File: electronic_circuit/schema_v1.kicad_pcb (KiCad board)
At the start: 2 copper layers, 74.2 x 51.8 mm, 34 parts, among them J1 Screw_Terminal_1x02, Q1 BC547, Q2 BC547, Q3 BC547, Q4 BC547, U1 MosfetIRF, U2 MosfetIRF, U3 STM32-Nucleo_Pinout, U4 MosfetIRF, U5 MosfetIRF, U6 mrf24j40ma, U7 DS-001

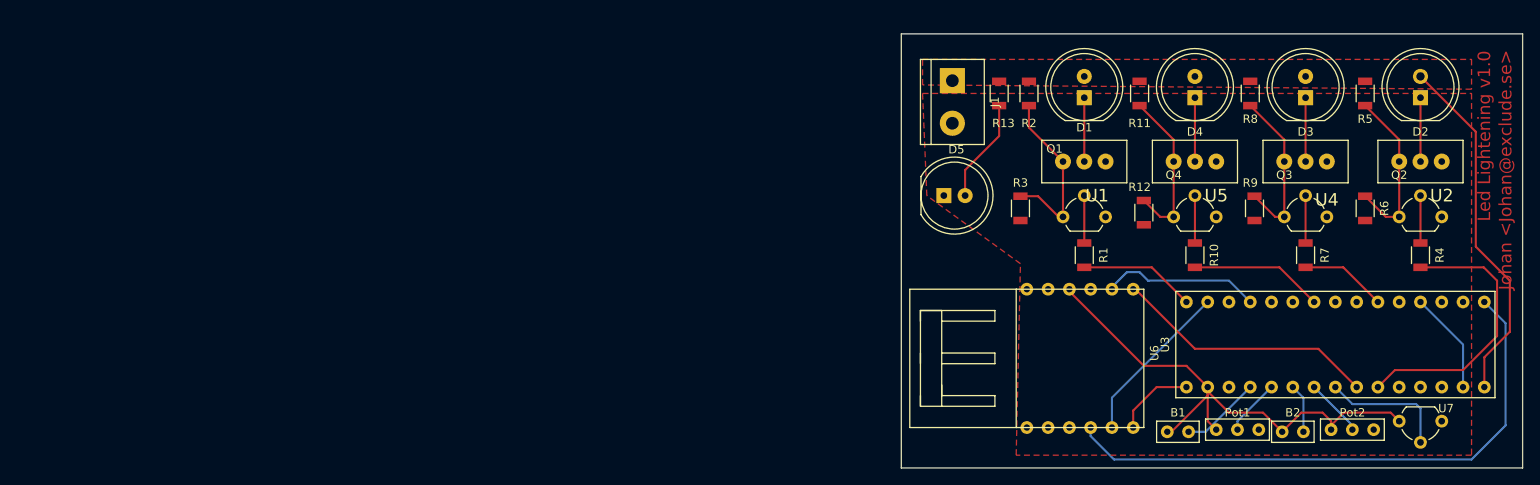
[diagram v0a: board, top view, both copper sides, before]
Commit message: New electronic schema
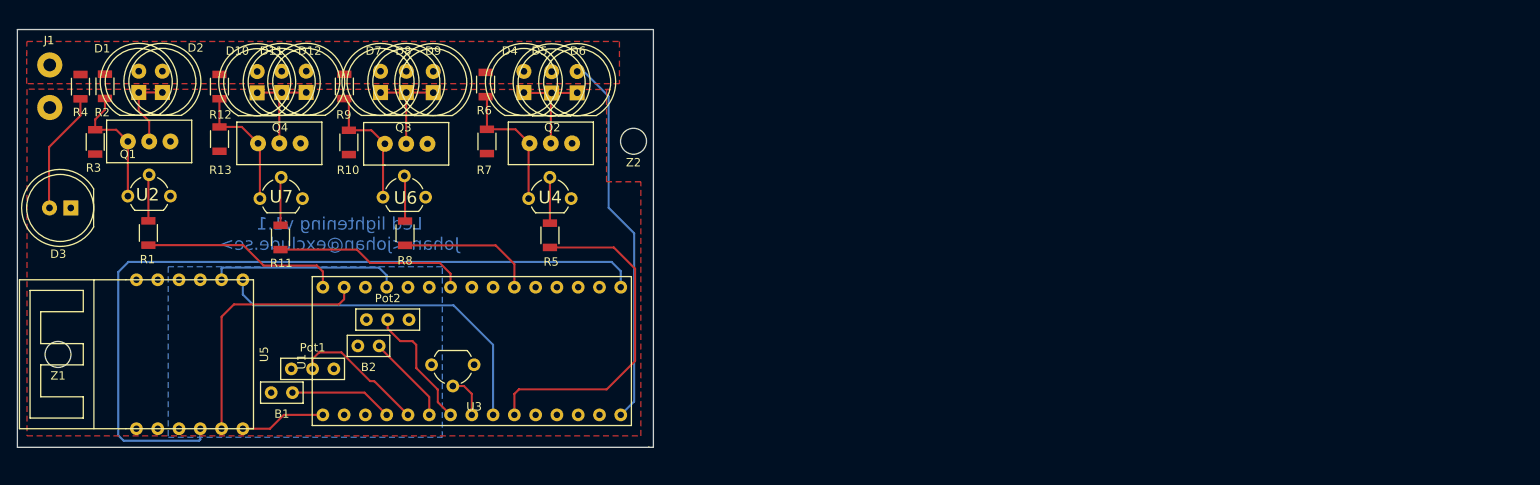
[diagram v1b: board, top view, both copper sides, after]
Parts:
- added D10: LED, LEDs:LED-8MM, F.Cu at (63.3, 30.4)
- added D11: LED, LEDs:LED-8MM, F.Cu at (69.2, 30.4)
- added D12: LED, LEDs:LED-8MM, F.Cu at (66.2, 30.4)
- added D6: LED, LEDs:LED-8MM, F.Cu at (101.5, 30.4)
- added D7: LED, LEDs:LED-8MM, F.Cu at (78.0, 30.4)
- added D8: LED, LEDs:LED-8MM, F.Cu at (81.1, 30.4)
- added D9: LED, LEDs:LED-8MM, F.Cu at (84.3, 30.4)
- added Z1: Drill_Hole, DrillHole:Drill_Hole, F.Cu at (39.5, 59.1)
- added Z2: Drill_Hole, DrillHole:Drill_Hole, F.Cu at (108.2, 33.6)
- J1: footprint Connectors:bornier2 -> potHoles:P_Led_Holes
- R10, R7: value 1k -> 39k
- R11, R5, R8: value 12k -> 1k
- R12, R6, R9: value 39k -> 12k
- R13: value 12k -> 39k
- R4: value 1k -> 12k
- U1: value MosfetIRF -> STM32-Nucleo_Pinout; footprint library:IRF3205 -> stm32nucleo:STM32-Nucleo_Pinout
- U3: value STM32-Nucleo_Pinout -> DS-001; footprint stm32nucleo:STM32-Nucleo_Pinout -> TO_SOT_Packages_THT:TO-92_Molded_Wide
- U5: value MosfetIRF -> mrf24j40ma; footprint library:IRF3205 -> mrf24j40ma:mrf24j40ma
- U6: value mrf24j40ma -> MosfetIRF; footprint mrf24j40ma:mrf24j40ma -> library:IRF3205
- U7: value DS-001 -> MosfetIRF; footprint TO_SOT_Packages_THT:TO-92_Molded_Wide -> library:IRF3205
- moved R4 161.2 mm to (42.2, 29.7)
- moved U2 151.8 mm to (47.9, 36.2)
- moved D2 150.2 mm to (52.0, 30.4)
- moved D3 148.0 mm to (41.1, 44.1), turned to 180 degrees
- moved U7 145.1 mm to (63.4, 36.4), turned to 0 degrees
- moved U5 139.7 mm to (34.9, 61.6), turned to 90 degrees
- moved U3 123.2 mm to (89.2, 62.9), turned to 180 degrees
- moved Pot2 115.4 mm to (78.9, 60.0), turned to 180 degrees
- moved D1 112.9 mm to (49.2, 30.4)
- moved R1 111.8 mm to (50.3, 47.1)
- moved Q1 111.7 mm to (47.9, 42.7)
- moved R12 111.4 mm to (58.8, 29.7)
- moved B2 110.8 mm to (76.6, 59.3)
- moved R3 110.7 mm to (44.0, 36.3)
- moved Pot1 110.4 mm to (69.9, 65.9), turned to 180 degrees
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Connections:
- D2 pad 1: Net-(D2-Pad1) -> Net-(D1-Pad1)
- D3 pad 1: Net-(D3-Pad1) -> GNDREF
- D3 pad 2: 12V -> Net-(D3-Pad2)
- D5 pad 1: GNDREF -> Net-(D4-Pad1)
- D5 pad 2: Net-(D5-Pad2) -> 12V
- R10 pad 1: Net-(Q4-Pad2) -> Net-(Q3-Pad1)
- R10 pad 2: RGB_B -> GNDREF
- R11 pad 1: 12V -> Net-(Q4-Pad2)
- R11 pad 2: Net-(Q4-Pad1) -> RGB_B
- R12 pad 1: Net-(Q4-Pad1) -> 12V
- R12 pad 2: GNDREF -> Net-(Q4-Pad1)
- R13 pad 1: 12V -> Net-(Q4-Pad1)
- R13 pad 2: Net-(D5-Pad2) -> GNDREF
- R4 pad 1: Net-(Q2-Pad2) -> 12V
- R4 pad 2: RGB_R -> Net-(D3-Pad2)
- R5 pad 1: 12V -> Net-(Q2-Pad2)
- R5 pad 2: Net-(Q2-Pad1) -> RGB_R
- R6 pad 1: Net-(Q2-Pad1) -> 12V
- R6 pad 2: GNDREF -> Net-(Q2-Pad1)
- R7 pad 1: Net-(Q3-Pad2) -> Net-(Q2-Pad1)
- R7 pad 2: RGB_G -> GNDREF
- R8 pad 1: 12V -> Net-(Q3-Pad2)
- R8 pad 2: Net-(Q3-Pad1) -> RGB_G
- R9 pad 1: Net-(Q3-Pad1) -> 12V
- R9 pad 2: GNDREF -> Net-(Q3-Pad1)
- U1 pad 1: Net-(Q1-Pad1) -> SPI_INT
- U1 pad 2: Net-(D1-Pad1) -> Net-(U1-Pad2)
- U1 pad 3: GNDREF -> Net-(U1-Pad3)
- U2 pad 1: Net-(Q2-Pad1) -> Net-(Q1-Pad1)
- U2 pad 2: Net-(D2-Pad1) -> Net-(D1-Pad1)
- U3 pad 1: SPI_INT -> GNDREF
- U3 pad 2: Net-(U3-Pad2) -> TEMP_SENSOR
- U3 pad 3: Net-(U3-Pad3) -> 3.3V
- U4 pad 1: Net-(Q3-Pad1) -> Net-(Q2-Pad1)
- U4 pad 2: Net-(D3-Pad1) -> Net-(D4-Pad1)
- U5 pad 1: Net-(Q4-Pad1) -> GNDREF
- U5 pad 2: Net-(D4-Pad1) -> MRF_RESET
- U5 pad 3: GNDREF -> Net-(U5-Pad3)
- U6 pad 1: GNDREF -> Net-(Q3-Pad1)
- U6 pad 3: MRF_RESET -> GNDREF
- U7 pad 1: GNDREF -> Net-(Q4-Pad1)
- U7 pad 2: TEMP_SENSOR -> Net-(D10-Pad1)
- U7 pad 3: 3.3V -> GNDREF
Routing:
- net 3.3V: track 63.9 -> 0.00 mm
- net SPI_INT: track 69.2 -> 93.8 mm
- net Net-(D3-Pad2): track 0.00 -> 14.6 mm
- net GNDREF: track 12.8 -> 0.00 mm
- net Net-(D5-Pad2): track 12.4 -> 0.00 mm
- net Net-(D7-Pad1): track 0.00 -> 12.4 mm
- net Net-(D10-Pad1): track 0.00 -> 12.0 mm
- net SPI_MISO: track 31.5 -> 42.5 mm
- net SPI_MOSI: track 19.7 -> 30.3 mm
- net TEMP_SENSOR: track 15.3 -> 5.16 mm
- net PANEL: track 13.9 -> 24.0 mm
- net Slider_1: track 6.76 -> 16.0 mm
- net Slider_2: track 6.97 -> 15.3 mm
- net Net-(D3-Pad1): track 7.62 -> 0.00 mm
- net Net-(D2-Pad1): track 7.62 -> 0.00 mm
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- added copper zone on B.Cu, net 3.3V
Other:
- board size 74.2 x 51.8 mm -> 75.9 x 49.9 mm
- board text added: "Led lightening v1.1 Johan <johan@exclude.se>"
- board text removed: "Johan <Johan@exclude.se>"
- board text removed: "Led Lightening v1.0"
